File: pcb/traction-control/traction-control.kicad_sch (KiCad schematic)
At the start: 50 parts, among them J1 Conn_01x05_Socket, J2 Conn_01x04_Pin, J3 Conn_ARM_SWD_TagConnect_TC203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, J4 Screw_Terminal_01x06, J5 Conn_01x04_Pin, Q1 AO3400A, Q2 AO3401A, SW1 SW_Push, SW2 SW_Push, SW3 SW_Push, SW4 SW_Push, U1 AT24CS32-SSHM, U2 STM32F103C8Tx, U3 AMS1117-3.3, U4 TPS5430DDA, Y1 16MHz

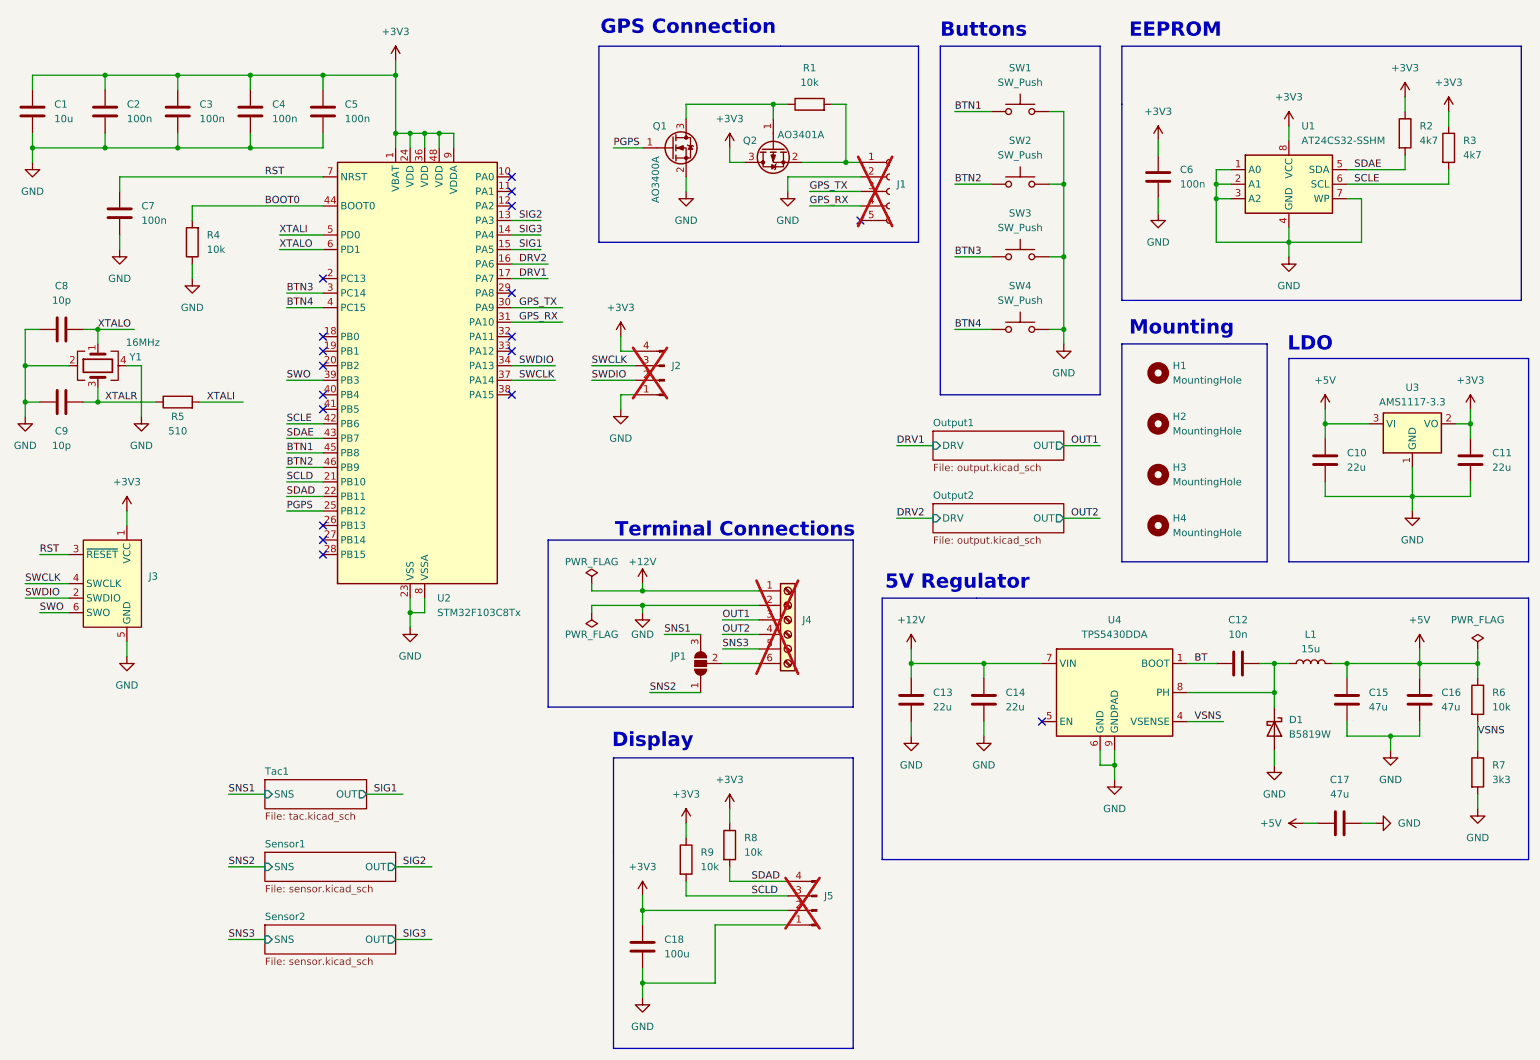
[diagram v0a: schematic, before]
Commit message: Make production files
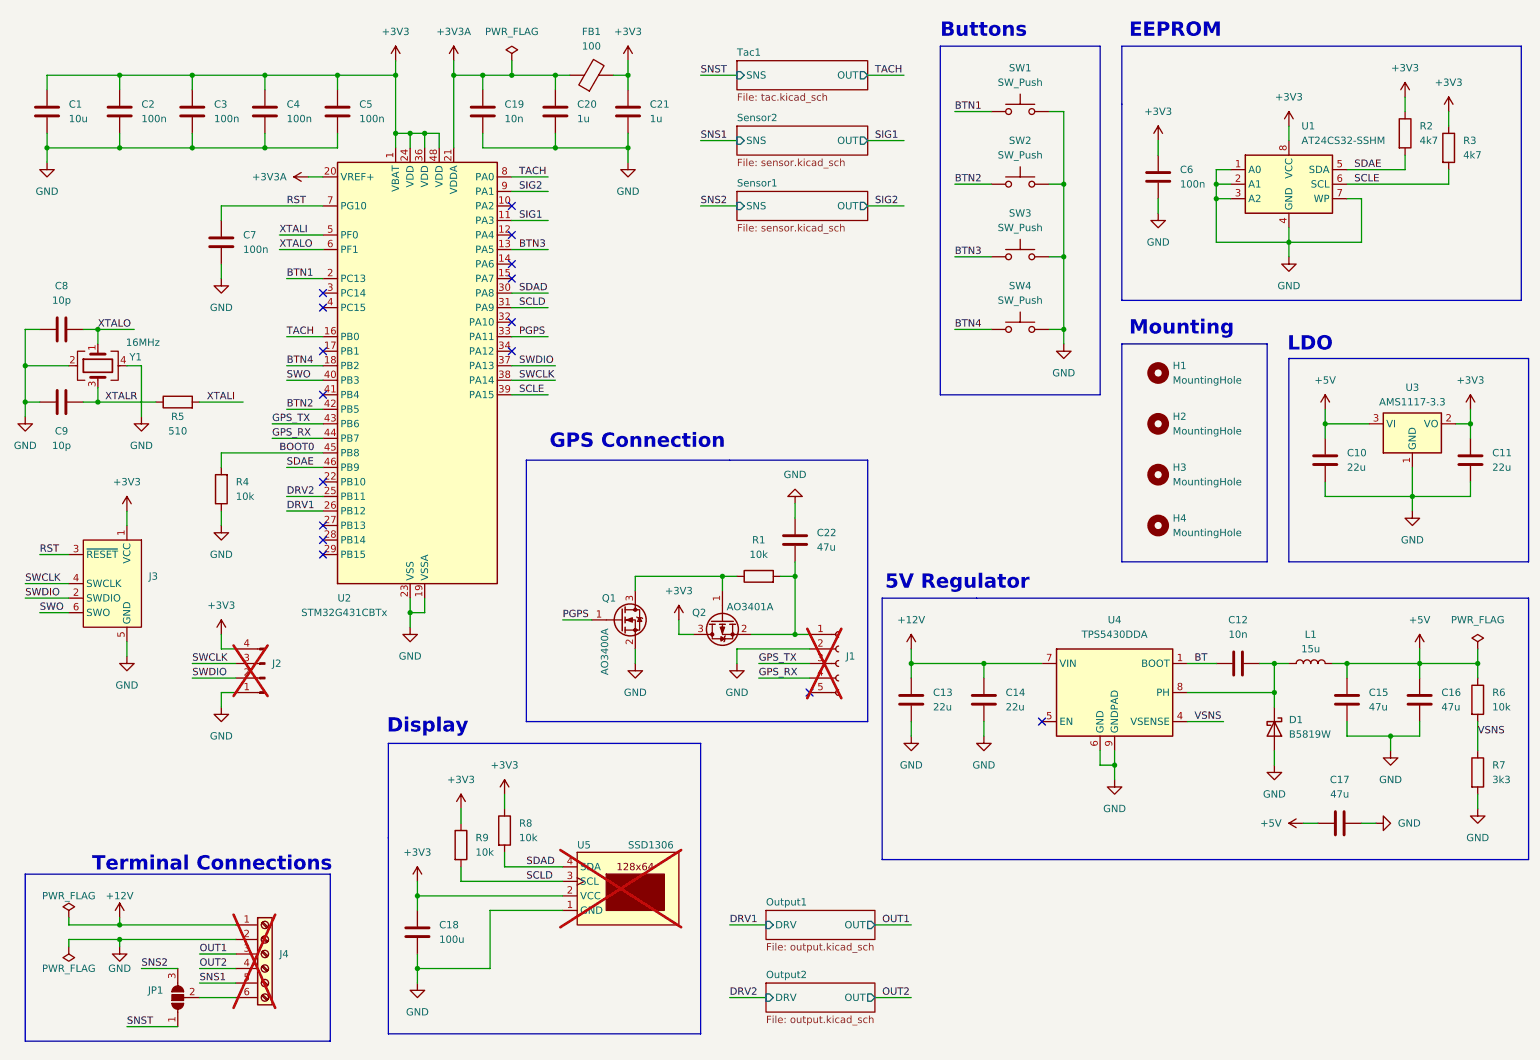
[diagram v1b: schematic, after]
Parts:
- removed J5: Conn_01x04_Pin, Connector_PinHeader_2.54mm:PinHeader_1x04_P2.54mm_Vertical, symbol Connector:Conn_01x04_Pin
- removed U2: STM32F103C8Tx, Package_QFP:LQFP-48_7x7mm_P0.5mm, symbol MCU_ST_STM32F1:STM32F103C8Tx
- added C19: 10n, Capacitor_SMD:C_0402_1005Metric, symbol Device:C
- added C20, C21: 1u, Capacitor_SMD:C_0402_1005Metric, symbol Device:C
- added C22: 47u, Capacitor_SMD:C_1206_3216Metric, symbol Device:C
- added FB1: 100, Inductor_SMD:L_0805_2012Metric, symbol Device:FerriteBead
- added U2: STM32G431CBTx, Package_QFP:LQFP-48_7x7mm_P0.5mm, symbol MCU_ST_STM32G4:STM32G431CBTx
- added U5: SSD1306, User_Footprints:SSD1309_1.3, symbol User_Symbols:SSD1306_128x64
- C2, C3, C4, C5, C7: LCSC (none) -> C1525
- C8, C9: LCSC (none) -> C32949
- J4: footprint TerminalBlock:TerminalBlock_bornier-6_P5.08mm -> User_Footprints:ScrewTerminalPlug_6P_P5.08
- R3: LCSC (none) -> C25900
- R4, R8, R9: LCSC (none) -> C25744
- Y1: LCSC (none) -> C13738
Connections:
- net SNS3 is gone; now on net SNS1: J4.5 (Pin_5)
- net +3V3: now also C21.1, FB1.2, U2.1 (VBAT), U2.24 (VDD), U2.36 (VDD), U2.48 (VDD), U5.2 (VCC)
- net BOOT0: now also U2.45 (PB8)
- net BTN1: now also U2.2 (PC13)
- net BTN2: now also U2.42 (PB5)
- net BTN3: now also U2.13 (PA5)
- net BTN4: now also U2.18 (PB2)
- net DRV1: now also U2.26 (PB12)
- net DRV2: now also U2.25 (PB11)
- net GND: now also C19.2, C20.2, C21.2, C22.2, U2.19 (VSSA), U2.23 (VSS), U2.35 (VSS), U2.47 (VSS), U5.1 (GND)
- net GPS_RX: now also U2.44 (PB7)
- net GPS_TX: now also U2.43 (PB6)
- net PGPS: now also U2.33 (PA11)
- net RST: now also U2.7 (PG10)
- net SCLD: now also U2.31 (PA9), U5.3 (SCL)
- net SCLE: now also U2.39 (PA15)
- net SDAD: now also U2.30 (PA8), U5.4 (SDA)
- net SDAE: now also U2.46 (PB9)
- net SIG1: now also U2.11 (PA3)
- net SIG2: now also U2.9 (PA1)
- net SNS1: no longer JP1.3 (B)
- net SNS2: now also JP1.3 (B); no longer JP1.1 (A)
- net SWCLK: now also U2.38 (PA14)
- net SWDIO: now also U2.37 (PA13)
- net SWO: now also U2.40 (PB3)
- net XTALI: now also U2.5 (PF0)
- net XTALO: now also U2.6 (PF1)
- net at J1.1 (Pin_1), Q2.2 (S), R1.2: now also C22.1
- new net +3V3A: C19.1, C20.1, FB1.1, U2.20 (VREF+), U2.21 (VDDA)
- new net SNST: JP1.1 (A)
- new net TACH: U2.16 (PB0), U2.8 (PA0)
- no-connect marks 18 -> 16
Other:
- moved on the sheet: C1, C18, C2, C3, C4, C5, J1, J2, J4, JP1, Q1, Q2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
